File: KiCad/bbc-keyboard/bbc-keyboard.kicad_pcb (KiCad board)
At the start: 2 copper layers, 337.8 x 137.2 mm, 101 parts, among them IC1 74LS161, IC2 74251, IC3 74145, IC4 74LS30, SW1 escape, SW10 W, SW11 2, SW12 A, SW13 S, SW14 Z, SW15 f2, SW16 4, SW17 E, SW18 D, SW19 X, SW2 Q, SW20 C, SW21 space, SW22 f3, SW23 5, SW24 T, SW25 R, SW26 F, SW27 G, SW28 V, SW29 f5, SW3 F0, SW30 F4, SW31 7, SW32 6, SW33 Y, SW34 H, SW35 B, SW36 f6, SW37 8, SW38 9, SW39 U, SW4 1, SW40 J, SW41 N, SW42 M, SW43 f8, SW44 f7, SW45 I, SW46 O, SW47 K, SW48 L, SW49 <,, SW5 caps lk, SW50 f9, SW51 =-, SW52 0, SW53 P, SW54 @, SW55 ;+, SW56 >., SW57 \|, SW58 ~^, SW59 _£, SW6 shift lk, SW60 {[, SW61 *:, SW62 }], SW63 ?/, SW64 right, SW65 left, SW66 down, SW67 up, SW68 return, SW69 delete, SW7 tab, SW70 copy, SW71 shift, SW72 shift, SW73 ctrl, SW74 SW_DIP_x08, SW75 break, SW8 f1, SW9 3

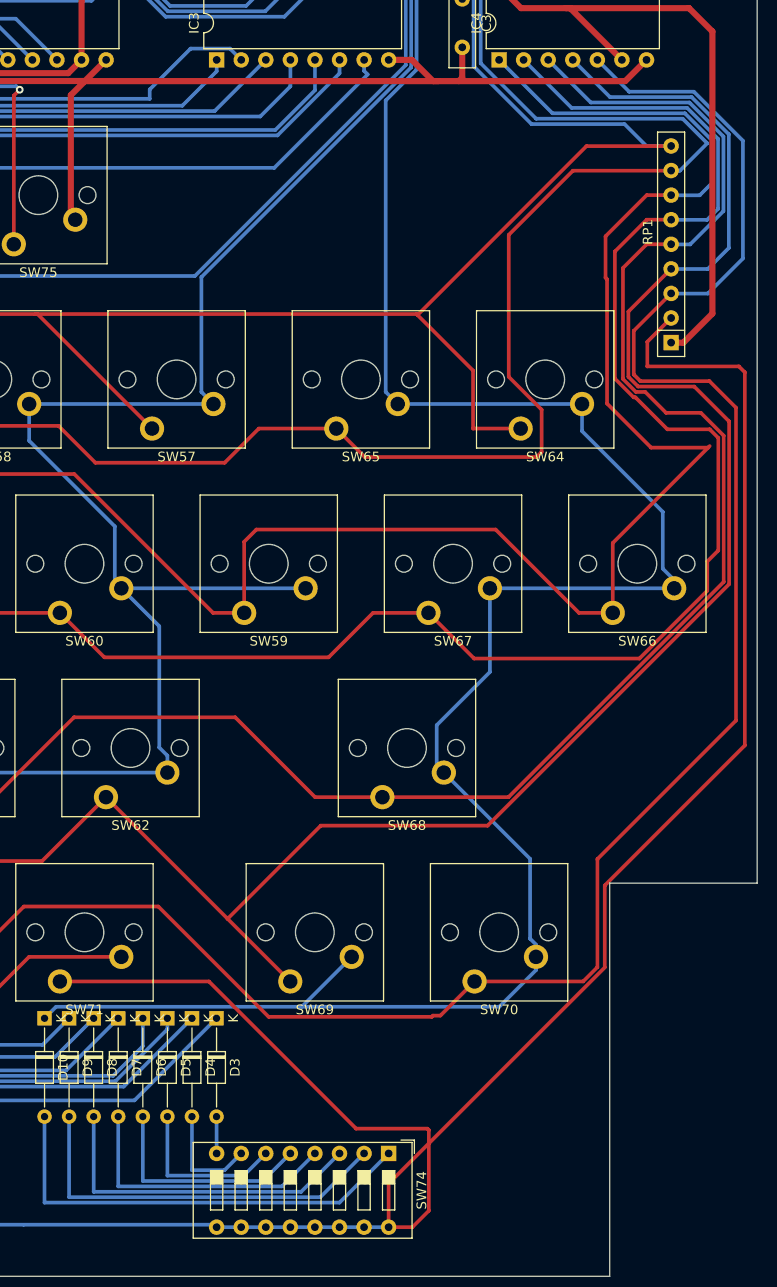
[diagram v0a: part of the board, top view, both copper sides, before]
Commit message: tidy routing
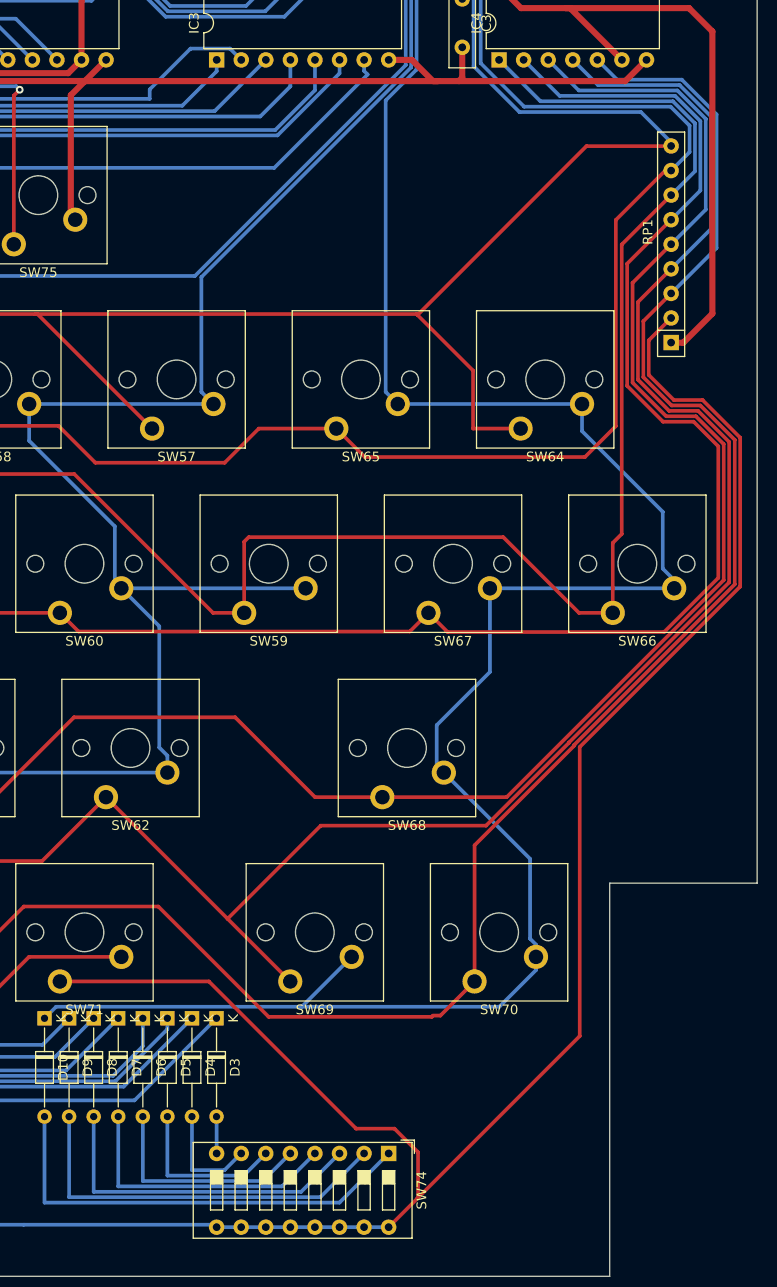
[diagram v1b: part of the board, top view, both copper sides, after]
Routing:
- net /Key Matrix/KC_ROW2: track 446.5 -> 428.6 mm
- net /Key Matrix/KC_ROW6: track 545.0 -> 530.5 mm
- net /Key Matrix/KC_ROW0: track 464.3 -> 451.5 mm
- net /Key Matrix/KC_ROW3: track 571.6 -> 559.9 mm
- net /Key Matrix/KC_ROW1: track 442.7 -> 435.2 mm
- net /Key Matrix/KC_ROW5: track 477.7 -> 471.4 mm
- net /Key Matrix/KC_ROW4: track 577.8 -> 571.9 mm
